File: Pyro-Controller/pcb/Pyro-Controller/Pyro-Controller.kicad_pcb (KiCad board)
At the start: 2 copper layers, 26.9 x 26.9 mm, 14 parts, among them J1 Screw_Terminal_01x02, J2 Conn_01x03_Socket, Q1 SiS454DN

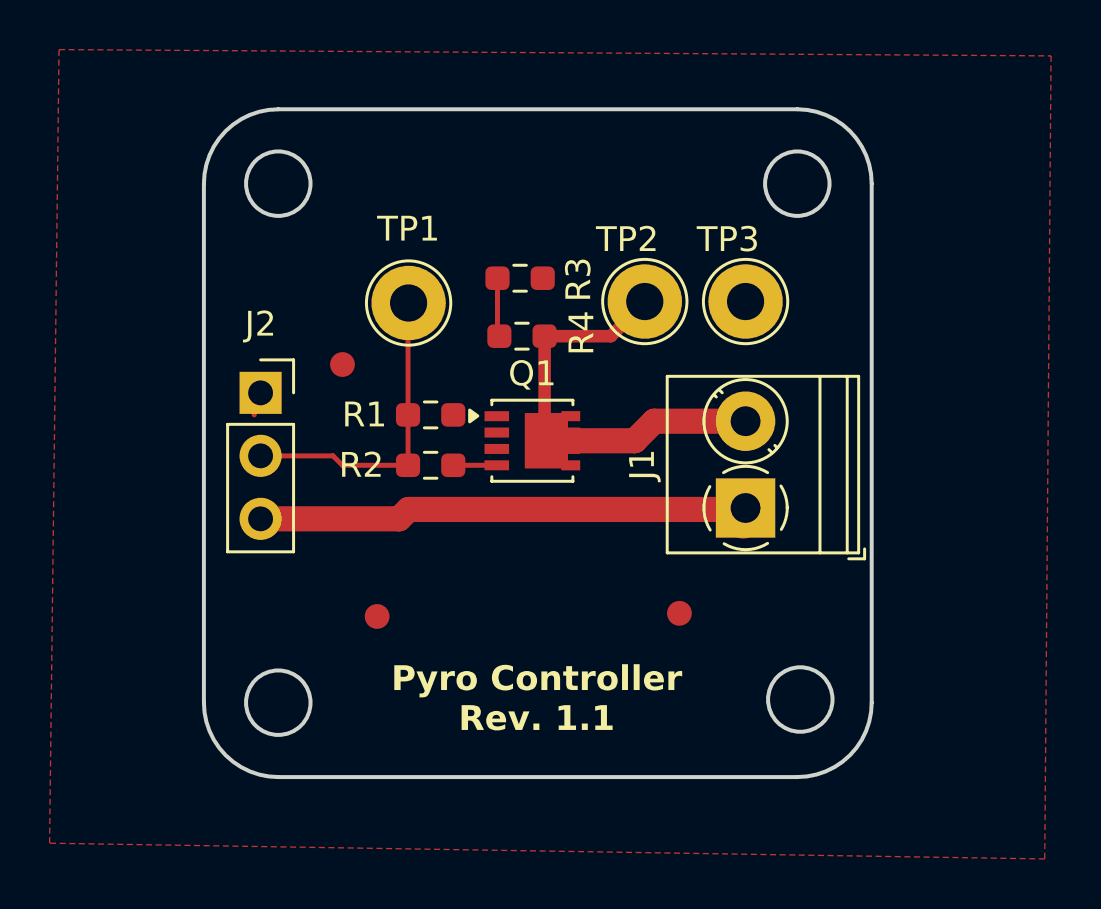
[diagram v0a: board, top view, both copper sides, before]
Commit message: Revert "Resolved recovery dev merge"
This reverts commit 81c4bbda93894cf9b120906f02d3dbab6bbd1e60, reversing
changes made to 220360569fc6c62025a0e7a68270d7f77f4a1f37.
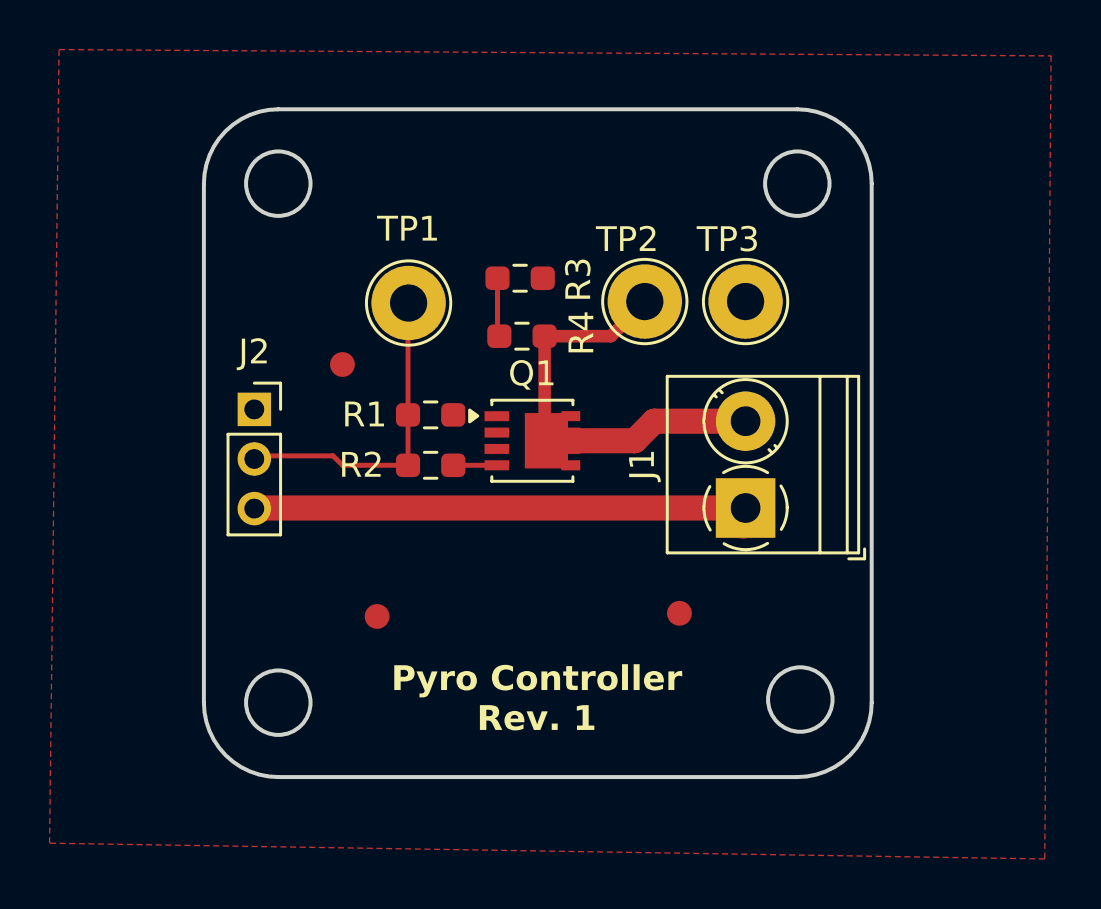
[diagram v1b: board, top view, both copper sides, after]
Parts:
- J2: footprint Connector_PinSocket_2.54mm:PinSocket_1x03_P2.54mm_Vertical -> Connector_PinSocket_2.00mm:PinSocket_1x03_P2.00mm_Vertical
- moved J2 0.71 mm to (25.7, 29.6)
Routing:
- net +3.3V: track 20.9 -> 20.4 mm
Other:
- board text added: "Pyro Controller Rev. 1"
- board text removed: "Pyro Controller Rev. 1.1"
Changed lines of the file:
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@@
 		)
 	)
-	(footprint "Connector_PinSocket_2.54mm:PinSocket_1x03_P2.54mm_Vertical"
+	(footprint "Connector_PinSocket_2.00mm:PinSocket_1x03_P2.00mm_Vertical"
 		(layer "F.Cu")
-		(at 25.908 28.956)
-		(descr "Through hole straight socket strip, 1x03, 2.54mm pitch, single row (from Kicad 4.0.7), script generated")
-		(tags "Through hole socket strip THT 1x03 2.54mm single row")
+		(at 25.654 29.623)
+		(descr "Through hole straight socket strip, 1x03, 2.00mm pitch, single row (from Kicad 4.0.7), script generated")
+		(tags "Through hole socket strip THT 1x03 2.00mm single row")
 		(property "Reference" "J2"
-			(at 0 -2.77 0)
+			(at 0 -2.318 0)
 			(layer "F.SilkS")
 			(effects
@@
 		)
 		(property "Value" "Conn_01x03_Socket"
-			(at 0 7.85 0)
+			(at 0 6.5 0)
 			(layer "F.Fab")
 			(effects
@@
 			)
 		)
-		(property "Footprint" "Connector_PinSocket_2.54mm:PinSocket_1x03_P2.54mm_Vertical"
+		(property "Footprint" "Connector_PinSocket_2.00mm:PinSocket_1x03_P2.00mm_Vertical"
 			(at 0 0 0)
 			(unlocked yes)
@@
 		(attr through_hole)
 		(fp_line
-			(start -1.33 1.27)
-			(end -1.33 6.41)
+			(start -1.06 1)
+			(end -1.06 5.06)
 			(stroke
 				(width 0.12)
@@
 		)
 		(fp_line
-			(start -1.33 1.27)
-			(end 1.33 1.27)
+			(start -1.06 1)
+			(end 1.06 1)
 			(stroke
 				(width 0.12)
@@
 		)
 		(fp_line
-			(start -1.33 6.41)
-			(end 1.33 6.41)
+			(start -1.06 5.06)
+			(end 1.06 5.06)
 			(stroke
 				(width 0.12)
@@
 		)
 		(fp_line
-			(start 0 -1.33)
-			(end 1.33 -1.33)
+			(start 0 -1.06)
+			(end 1.06 -1.06)
 			(stroke
 				(width 0.12)
@@
 		)
 		(fp_line
-			(start 1.33 -1.33)
-			(end 1.33 0)
+			(start 1.06 -1.06)
+			(end 1.06 0)
 			(stroke
 				(width 0.12)
@@
 		)
 		(fp_line
-			(start 1.33 1.27)
-			(end 1.33 6.41)
+			(start 1.06 1)
+			(end 1.06 5.06)
 			(stroke
 				(width 0.12)
@@
 		)
 		(fp_line
-			(start -1.8 -1.8)
-			(end 1.75 -1.8)
+			(start -1.5 -1.5)
+			(end 1.5 -1.5)
 			(stroke
 				(width 0.05)
@@
 		)
 		(fp_line
-			(start -1.8 6.85)
-			(end -1.8 -1.8)
+			(start -1.5 5.5)
+			(end -1.5 -1.5)
 			(stroke
 				(width 0.05)
@@
 		)
 		(fp_line
-			(start 1.75 -1.8)
-			(end 1.75 6.85)
+			(start 1.5 -1.5)
+			(end 1.5 5.5)
 			(stroke
 				(width 0.05)
@@
 		)
 		(fp_line
-			(start 1.75 6.85)
-			(end -1.8 6.85)
+			(start 1.5 5.5)
+			(end -1.5 5.5)
 			(stroke
 				(width 0.05)
@@
 		)
 		(fp_line
-			(start -1.27 -1.27)
-			(end 0.635 -1.27)
+			(start -1 -1)
+			(end 0.5 -1)
 			(stroke
 				(width 0.1)
@@
 		)
 		(fp_line
-			(start -1.27 6.35)
-			(end -1.27 -1.27)
+			(start -1 5)
+			(end -1 -1)
 			(stroke
 				(width 0.1)
@@
 		)
 		(fp_line
-			(start 0.635 -1.27)
-			(end 1.27 -0.635)
+			(start 0.5 -1)
+			(end 1 -0.5)
 			(stroke
 				(width 0.1)
@@
 		)
 		(fp_line
-			(start 1.27 -0.635)
-			(end 1.27 6.35)
+			(start 1 -0.5)
+			(end 1 5)
 			(stroke
 				(width 0.1)
@@
 		)
 		(fp_line
-			(start 1.27 6.35)
-			(end -1.27 6.35)
+			(start 1 5)
+			(end -1 5)
 			(stroke
 				(width 0.1)
@@
 		)
 		(fp_text user "${REFERENCE}"
-			(at 0 2.54 90)
+			(at 0 2 90)
 			(layer "F.Fab")
 			(effects
@@
 		(pad "1" thru_hole rect
 			(at 0 0)
-			(size 1.7 1.7)
-			(drill 1)
+			(size 1.35 1.35)
+			(drill 0.8)
 			(layers "*.Cu" "*.Mask")
 			(remove_unused_layers no)
@@
 		)
 		(pad "2" thru_hole oval
-			(at 0 2.54)
-			(size 1.7 1.7)
-			(drill 1)
+			(at 0 2)
+			(size 1.35 1.35)
+			(drill 0.8)
 			(layers "*.Cu" "*.Mask")
 			(remove_unused_layers no)
@@
 		)
 		(pad "3" thru_hole oval
-			(at 0 5.08)
-			(size 1.7 1.7)
-			(drill 1)
+			(at 0 4)
+			(size 1.35 1.35)
+			(drill 0.8)
 			(layers "*.Cu" "*.Mask")
 			(remove_unused_layers no)
@@
 			(pintype "passive")
 		)
-		(model "${KICAD8_3DMODEL_DIR}/Connector_PinSocket_2.54mm.3dshapes/PinSocket_1x03_P2.54mm_Vertical.wrl"
+		(model "${KICAD8_3DMODEL_DIR}/Connector_PinSocket_2.00mm.3dshapes/PinSocket_1x03_P2.00mm_Vertical.wrl"
 			(offset
 				(xyz 0 0 0)
@@
 		(layer "Edge.Cuts")
 	)
-	(gr_text "Pyro Controller\nRev. 1.1"
+	(gr_text "Pyro Controller\nRev. 1"
 		(at 37.043404 42.672 0)
 		(layer "B.SilkS")
@@
 		)
 	)
-	(gr_text "Pyro Controller\nRev. 1.1"
-		(at 37.043404 42.672 0)
+	(gr_text "Pyro Controller\nRev. 1"
+		(at 37.043404 42.672 -0)
 		(layer "F.SilkS")
 		(effects
@@
 	)
 	(segment
-		(start 31.496 34.036)
-		(end 25.679 34.036)
+		(start 45.466 33.599)
+		(end 25.964 33.599)
 		(width 1.016)
 		(layer "F.Cu")
@@
 	)
 	(segment
-		(start 31.87425 33.65775)
-		(end 31.496 34.036)
-		(width 1.016)
-		(layer "F.Cu")
-		(net 1)
-	)
-	(segment
-		(start 25.679 34.036)
-		(end 25.679 33.884)
+		(start 25.964 33.599)
+		(end 25.908 33.655)
 		(width 1.016)
 		(layer "F.Cu")
@@
 		(width 1.016)
 		(layer "F.Cu")
-		(net 1)
-	)
-	(segment
-		(start 45.40725 33.65775)
-		(end 31.87425 33.65775)
-		(width 1.016)
-		(layer "F.Cu")
-		(net 1)
-	)
-	(segment
-		(start 45.466 33.599)
-		(end 45.40725 33.65775)
-		(width 1.016)
-		(layer "F.Cu")
